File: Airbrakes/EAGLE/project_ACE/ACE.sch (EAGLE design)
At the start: 4 parts, among them J3 PTH

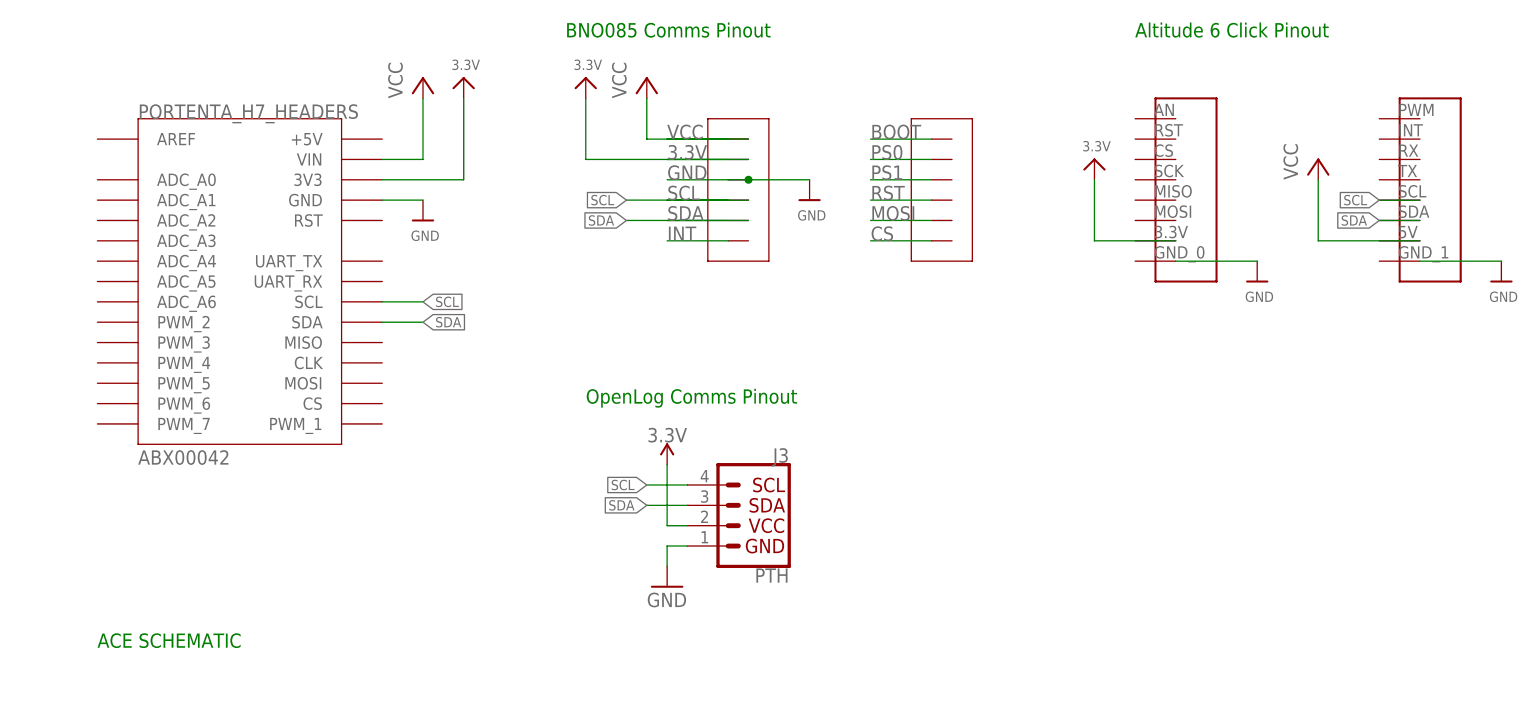
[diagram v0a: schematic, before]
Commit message: Update ACE.sch
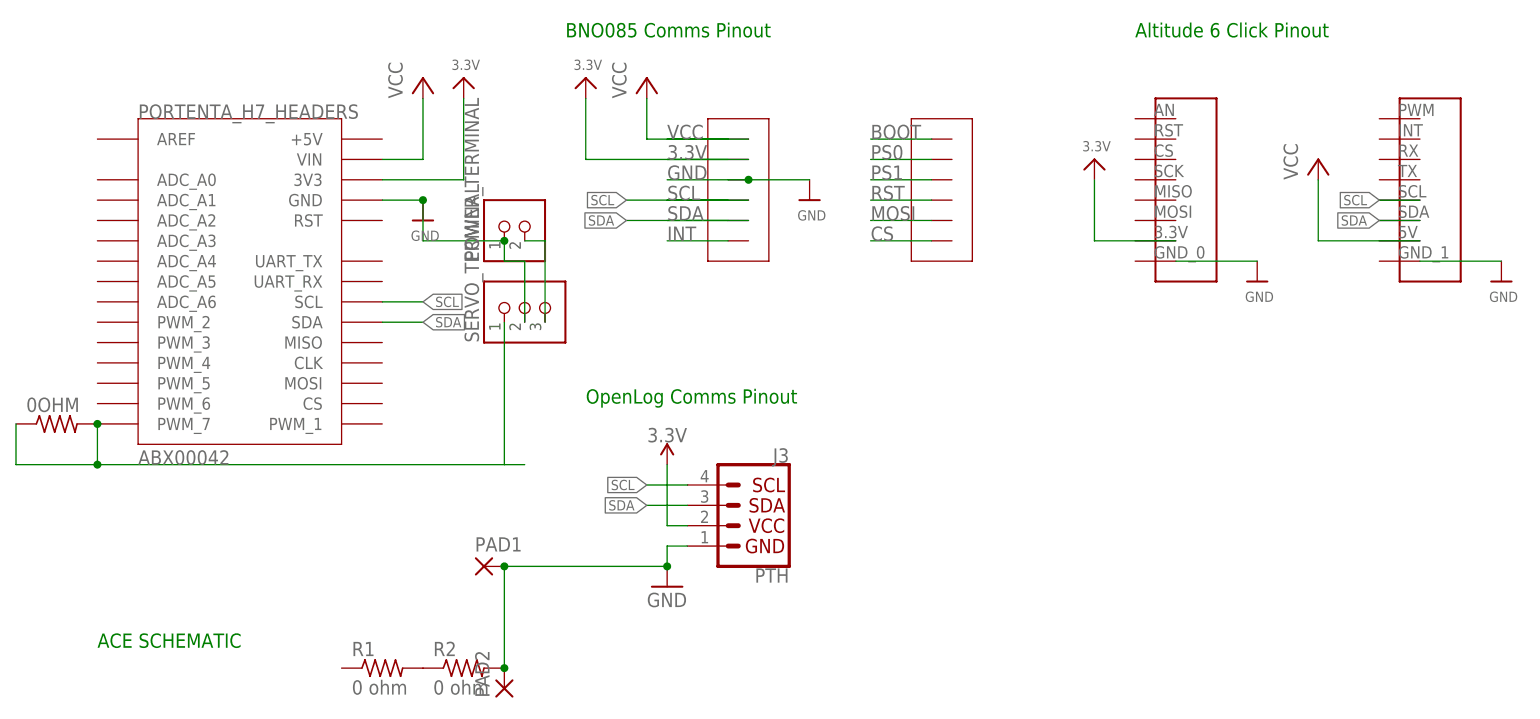
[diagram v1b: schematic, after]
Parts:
- added 0OHM: (no value), fab_new:R1206
- added PAD1, PAD2: (no value), wirepad:2,15/1,0
- added POWER_TERMINAL: CONN_02_TERM-ADAFRUIT, fab_new:CONN_02_TERM-ADAFRUIT
- added R1, R2: 0 ohm, fab_new:R1206
- added SERVO_TERMINAL: CONN_03_TERM'-FABLAB', fab_new:CONN_03_TERM'-FABLAB'
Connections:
- new net 7.4V: POWER_TERMINAL.2, SERVO_TERMINAL.3
- new net N$2: R1.2, R2.1
- new net PWM: 0OHM.1, 0OHM.2, SERVO_TERMINAL.1, U$10.PWM_7
- net GND: now also PAD1.P, PAD2.P, POWER_TERMINAL.1, R2.2, SERVO_TERMINAL.2
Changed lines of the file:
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@@
 <layers>
 <layer number="1" name="Top" color="4" fill="1" visible="no" active="no"/>
+<layer number="2" name="Route2" color="1" fill="3" visible="no" active="no"/>
+<layer number="3" name="Route3" color="4" fill="3" visible="no" active="no"/>
+<layer number="4" name="Route4" color="1" fill="4" visible="no" active="no"/>
+<layer number="5" name="Route5" color="4" fill="4" visible="no" active="no"/>
+<layer number="6" name="Route6" color="1" fill="8" visible="no" active="no"/>
+<layer number="7" name="Route7" color="4" fill="8" visible="no" active="no"/>
+<layer number="8" name="Route8" color="1" fill="2" visible="no" active="no"/>
+<layer number="9" name="Route9" color="4" fill="2" visible="no" active="no"/>
+<layer number="10" name="Route10" color="1" fill="7" visible="no" active="no"/>
+<layer number="11" name="Route11" color="4" fill="7" visible="no" active="no"/>
+<layer number="12" name="Route12" color="1" fill="5" visible="no" active="no"/>
+<layer number="13" name="Route13" color="4" fill="5" visible="no" active="no"/>
+<layer number="14" name="Route14" color="1" fill="6" visible="no" active="no"/>
+<layer number="15" name="Route15" color="4" fill="6" visible="no" active="no"/>
 <layer number="16" name="Bottom" color="1" fill="1" visible="no" active="no"/>
 <layer number="17" name="Pads" color="2" fill="1" visible="no" active="no"/>
@@
 <part name="P+1" library="supply1" library_urn="urn:adsk.eagle:library:371" deviceset="VCC" device=""/>
 <part name="U$12" library="microbuilder" deviceset="GND" device=""/>
+<part name="R1" library="fab_new" deviceset="R" device="1206" value="0 ohm"/>
+<part name="R2" library="fab_new" deviceset="R" device="1206" value="0 ohm"/>
+<part name="POWER_TERMINAL" library="fab_new" deviceset="CONN_02_TERM" device="-ADAFRUIT"/>
+<part name="SERVO_TERMINAL" library="fab_new" deviceset="CONN_03_TERM" device="'-FABLAB'"/>
+<part name="0OHM" library="fab_new" deviceset="R" device="1206"/>
+<part name="PAD1" library="wirepad" library_urn="urn:adsk.eagle:library:412" deviceset="2,15/1,0" device="" package3d_urn="urn:adsk.eagle:package:30831/1"/>
+<part name="PAD2" library="wirepad" library_urn="urn:adsk.eagle:library:412" deviceset="2,15/1,0" device="" package3d_urn="urn:adsk.eagle:package:30831/1"/>
 </parts>
 <sheets>
@@
 <attribute name="VALUE" x="39.116" y="55.88" size="1.27" layer="96"/>
 </instance>
+<instance part="R1" gate="G$1" x="35.56" y="2.54" smashed="yes">
+<attribute name="NAME" x="31.75" y="4.0386" size="1.778" layer="95"/>
+<attribute name="VALUE" x="31.75" y="-0.762" size="1.778" layer="96"/>
+</instance>
+<instance part="R2" gate="G$1" x="45.72" y="2.54" smashed="yes">
+<attribute name="NAME" x="41.91" y="4.0386" size="1.778" layer="95"/>
+<attribute name="VALUE" x="41.91" y="-0.762" size="1.778" layer="96"/>
+</instance>
+<instance part="POWER_TERMINAL" gate="G$1" x="53.34" y="55.88" smashed="yes" rot="R90">
+<attribute name="NAME" x="47.625" y="53.34" size="1.778" layer="95" rot="R90"/>
+</instance>
+<instance part="SERVO_TERMINAL" gate="G$1" x="53.34" y="45.72" smashed="yes" rot="R90">
+<attribute name="NAME" x="47.625" y="43.18" size="1.778" layer="95" rot="R90"/>
+</instance>
+<instance part="0OHM" gate="G$1" x="-5.08" y="33.02" smashed="yes">
+<attribute name="NAME" x="-8.89" y="34.5186" size="1.778" layer="95"/>
+<attribute name="VALUE" x="-8.89" y="29.718" size="1.778" layer="96"/>
+</instance>
+<instance part="PAD1" gate="1" x="48.26" y="15.24" smashed="yes">
+<attribute name="NAME" x="47.117" y="17.0942" size="1.778" layer="95"/>
+<attribute name="VALUE" x="47.117" y="11.938" size="1.778" layer="96"/>
+</instance>
+<instance part="PAD2" gate="1" x="50.8" y="0" smashed="yes" rot="R90">
+<attribute name="NAME" x="48.9458" y="-1.143" size="1.778" layer="95" rot="R90"/>
+<attribute name="VALUE" x="54.102" y="-1.143" size="1.778" layer="96" rot="R90"/>
+</instance>
 </instances>
 <busses>
@@
 <wire x1="71.12" y1="17.78" x2="71.12" y2="15.24" width="0.1524" layer="91"/>
 <pinref part="GND12" gate="1" pin="GND"/>
+<pinref part="R2" gate="G$1" pin="2"/>
+<wire x1="71.12" y1="15.24" x2="50.8" y2="15.24" width="0.1524" layer="91"/>
+<wire x1="50.8" y1="15.24" x2="50.8" y2="2.54" width="0.1524" layer="91"/>
+<junction x="71.12" y="15.24"/>
+<pinref part="PAD1" gate="1" pin="P"/>
+<junction x="50.8" y="15.24"/>
+<pinref part="PAD2" gate="1" pin="P"/>
+<junction x="50.8" y="2.54"/>
 </segment>
 <segment>
@@
 <wire x1="35.56" y1="60.96" x2="40.64" y2="60.96" width="0.1524" layer="91"/>
 <pinref part="U$10" gate="G$1" pin="GND"/>
+<wire x1="40.64" y1="60.96" x2="40.64" y2="55.88" width="0.1524" layer="91"/>
+<junction x="40.64" y="60.96"/>
+<pinref part="POWER_TERMINAL" gate="G$1" pin="1"/>
+<wire x1="40.64" y1="55.88" x2="50.8" y2="55.88" width="0.1524" layer="91"/>
+<pinref part="SERVO_TERMINAL" gate="G$1" pin="2"/>
+<wire x1="53.34" y1="45.72" x2="53.34" y2="53.34" width="0.1524" layer="91"/>
+<wire x1="53.34" y1="53.34" x2="50.8" y2="53.34" width="0.1524" layer="91"/>
+<wire x1="50.8" y1="53.34" x2="50.8" y2="55.88" width="0.1524" layer="91"/>
+<junction x="50.8" y="55.88"/>
 </segment>
 </net>
@@
 <pinref part="U$1" gate="G$1" pin="GND_1"/>
 <wire x1="165.1" y1="53.34" x2="175.26" y2="53.34" width="0.1524" layer="91"/>
+</segment>
+</net>
+<net name="N$2" class="0">
+<segment>
+<pinref part="R1" gate="G$1" pin="2"/>
+<pinref part="R2" gate="G$1" pin="1"/>
+</segment>
+</net>
+<net name="7.4V" class="0">
+<segment>
+<pinref part="POWER_TERMINAL" gate="G$1" pin="2"/>
+<pinref part="SERVO_TERMINAL" gate="G$1" pin="3"/>
+<wire x1="53.34" y1="55.88" x2="55.88" y2="55.88" width="0.1524" layer="91"/>
+<wire x1="55.88" y1="55.88" x2="55.88" y2="45.72" width="0.1524" layer="91"/>
+</segment>
+</net>
+<net name="PWM" class="0">
+<segment>
+<pinref part="0OHM" gate="G$1" pin="1"/>
+<wire x1="-10.16" y1="33.02" x2="-10.16" y2="27.94" width="0.1524" layer="91"/>
+<wire x1="-10.16" y1="27.94" x2="0" y2="27.94" width="0.1524" layer="91"/>
+<pinref part="SERVO_TERMINAL" gate="G$1" pin="1"/>
+<wire x1="0" y1="27.94" x2="50.8" y2="27.94" width="0.1524" layer="91"/>
+<wire x1="53.34" y1="27.94" x2="50.8" y2="27.94" width="0.1524" layer="91"/>
+<wire x1="50.8" y1="27.94" x2="50.8" y2="45.72" width="0.1524" layer="91"/>
+<pinref part="U$10" gate="G$1" pin="PWM_7"/>
+<pinref part="0OHM" gate="G$1" pin="2"/>
+<wire x1="0" y1="33.02" x2="0" y2="27.94" width="0.1524" layer="91"/>
+<junction x="0" y="33.02"/>
+<junction x="0" y="27.94"/>
 </segment>
 </net>
@@
 will not be understood (or retained) with this version.
 </note>
+<note version="8.3" severity="warning">
+Since Version 8.3, EAGLE supports the association of 3D packages
+with devices in libraries, schematics, and board files. Those 3D
+packages will not be understood (or retained) with this version.
+</note>
 </compatibility>
